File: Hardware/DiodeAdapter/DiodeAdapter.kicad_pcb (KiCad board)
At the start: 2 copper layers, 83 x 78 mm, 305 parts, among them P1 LED, P2 LED, P3 LED, P4 LED, X01 CONN_01X02, X02 CONN_01X02, X1 CONN_01X02, X2 CONN_01X02, X3 CONN_01X02, X4 CONN_01X02, X5 CONN_01X02, X6 CONN_01X02

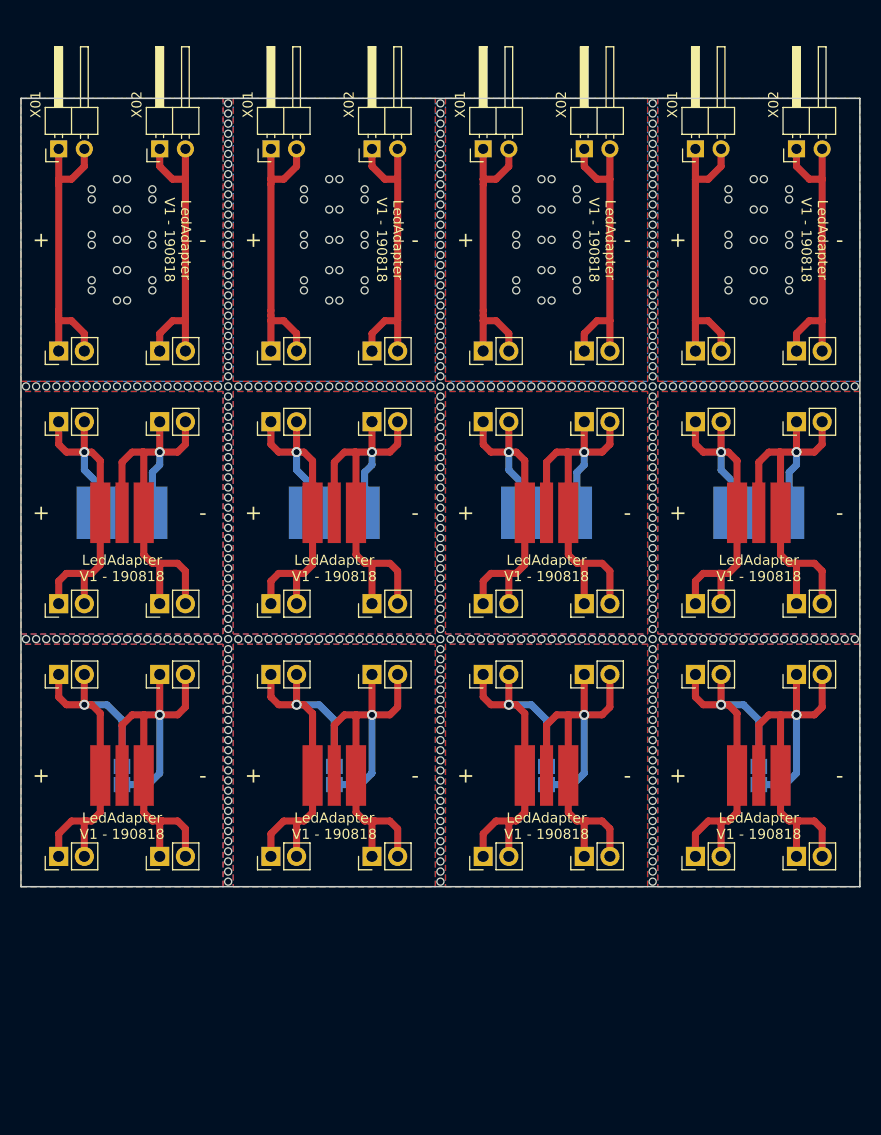
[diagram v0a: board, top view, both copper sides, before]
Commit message: Update for next version
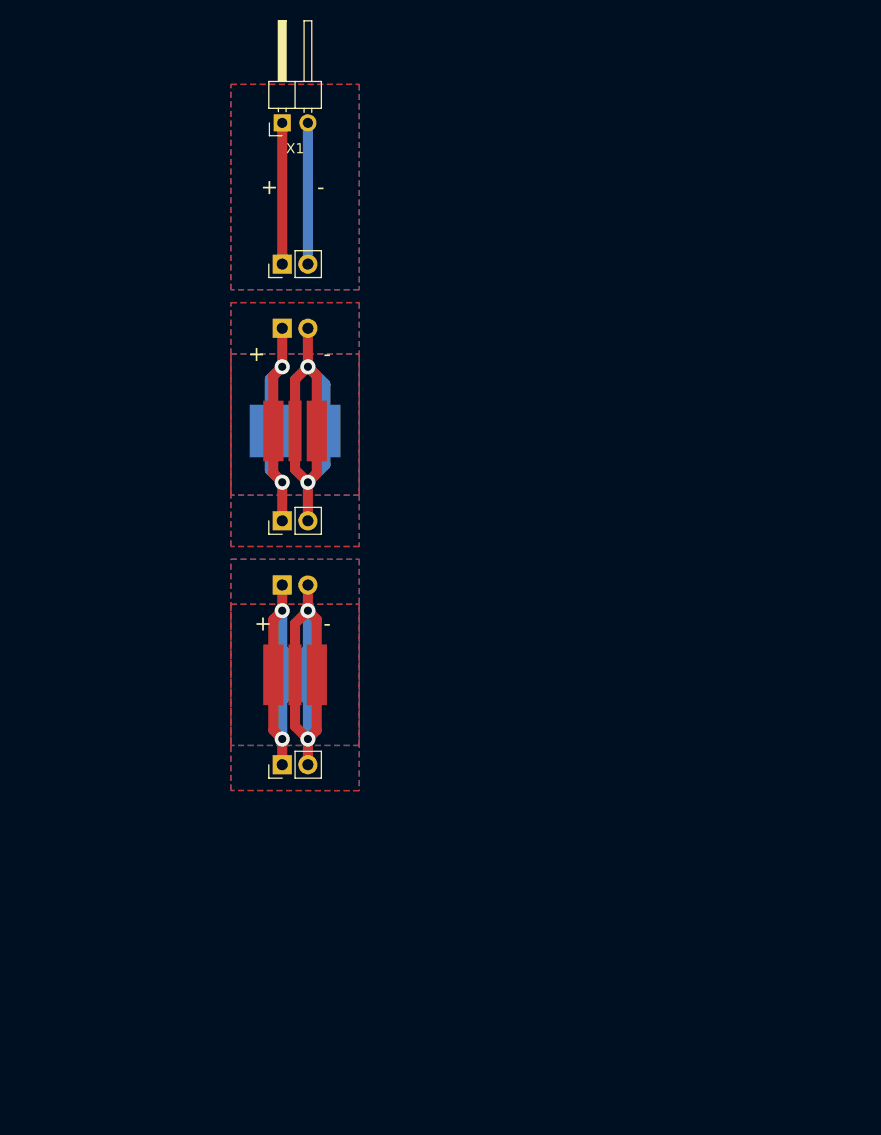
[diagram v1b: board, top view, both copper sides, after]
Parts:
- removed the P1 at (127.0, 87.0)
- removed the P1 at (106.0, 87.0)
- removed the P1 at (85.0, 87.0)
- removed the P1 at (64.0, 87.0)
- removed the P2 at (127.0, 87.0)
- removed the P2 at (106.0, 87.0)
- removed the P2 at (85.0, 87.0)
- removed the P2 at (64.0, 87.0)
- removed the P3 at (127.0, 113.0)
- removed the P3 at (106.0, 113.0)
- removed the P3 at (85.0, 113.0)
- removed the P3 at (64.0, 113.0)
- removed the P4 at (127.0, 113.0)
- removed the P4 at (106.0, 113.0)
- removed the P4 at (85.0, 113.0)
- removed the P4 at (64.0, 113.0)
- removed REF** (x241): BoardCutter_2, MyLib:BoardCutter_2
- removed X01 (x4), X02 (x4): CONN_01X02, MyLib:Pin_Header_Angled_1x02_Pitch2.54mm
- removed the X1 at (122.0, 71.0)
- removed the X1 at (101.0, 71.0)
- removed the X1 at (80.0, 71.0)
- removed the X1 at (59.0, 71.0)
- removed the X2 at (132.0, 71.0)
- removed the X2 at (111.0, 71.0)
- removed the X2 at (90.0, 71.0)
- removed the X2 at (69.0, 71.0)
- removed the X3 at (122.0, 78.0)
- removed the X3 at (122.0, 96.0)
- removed the X3 at (101.0, 96.0)
- removed the X3 at (101.0, 78.0)
- removed the X3 at (80.0, 78.0)
- removed the X3 at (80.0, 96.0)
- removed the X3 at (59.0, 96.0)
- removed the X3 at (59.0, 78.0)
- removed the X4 at (132.0, 78.0)
- removed the X4 at (132.0, 96.0)
- removed the X4 at (111.0, 96.0)
- removed the X4 at (111.0, 78.0)
- removed the X4 at (90.0, 78.0)
- removed the X4 at (90.0, 96.0)
- removed the X4 at (69.0, 96.0)
- removed the X4 at (69.0, 78.0)
- removed the X5 at (122.0, 103.0)
- removed the X5 at (122.0, 121.0)
- removed the X5 at (101.0, 121.0)
- removed the X5 at (101.0, 103.0)
- removed the X5 at (80.0, 103.0)
- removed the X5 at (80.0, 121.0)
- removed the X5 at (59.0, 121.0)
- removed the X5 at (59.0, 103.0)
- removed the X6 at (132.0, 103.0)
- removed the X6 at (132.0, 121.0)
- removed the X6 at (111.0, 121.0)
- removed the X6 at (111.0, 103.0)
- removed the X6 at (90.0, 103.0)
- removed the X6 at (90.0, 121.0)
- removed the X6 at (69.0, 121.0)
- removed the X6 at (69.0, 103.0)
- added P1: LED, 0EsseivaN_Lib:LED_LH351D, F.Cu at (81.1, 78.9)
- added P2: LED, 0EsseivaN_Lib:LED_LITTLE_STAR, B.Cu at (81.1, 78.9)
- added P3: LED, 0EsseivaN_Lib:LED_LH351D, F.Cu at (81.1, 103.0)
- added P4: LED, 0EsseivaN_Lib:LED_XQ_D, B.Cu at (81.1, 103.0)
- added X1: CONN_01X02, 0EsseivaN_Lib:Pin_Header_Angled_1x02_Pitch2.54mm, F.Cu at (81.1, 48.4)
- added X2: CONN_01X02, 0EsseivaN_Lib:Pin_Header_Straight_1x02_Pitch2.54mm, F.Cu at (81.1, 62.4)
- added X3: CONN_01X02, 0EsseivaN_Lib:Pin_Header_Straight_1x02_Pitch2.54mm, F.Cu at (81.1, 87.8)
- added X4: CONN_01X02, 0EsseivaN_Lib:Pin_Header_Straight_1x02_Pitch2.54mm, B.Cu at (81.1, 68.8)
- added X5: CONN_01X02, 0EsseivaN_Lib:Pin_Header_Straight_1x02_Pitch2.54mm, B.Cu at (81.1, 94.2)
- added X6: CONN_01X02, 0EsseivaN_Lib:Pin_Header_Straight_1x02_Pitch2.54mm, F.Cu at (81.1, 111.9)
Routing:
- net /GND_2: track 201.5 -> 45.3 mm, vias 4 -> 2
- net /GND_1: track 184.3 -> 45.1 mm, vias 4 -> 2
- net /V+_2: track 158.9 -> 31.5 mm, vias 4 -> 2
- net /V+_1: track 150.6 -> 32.2 mm, vias 4 -> 2
- net /V+: track 118.4 -> 14.0 mm
- net /GND: track 118.4 -> 14.0 mm
- added copper zone on F.Cu, net /GND_1
- added copper zone on F.Cu, net /GND_2
- removed copper zone on F.Cu, net /V+_1
- removed copper zone on F.Cu, net /V+_2
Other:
- board outline removed
- net class Default: trace_width 0.7 -> 1; via_dia 1 -> 1.5; via_drill 0.6 -> 0.8
- board text removed: "Holes to better stick with glue"
- board text removed: "LedAdapter V1 - 190818"

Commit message: Version 6 final
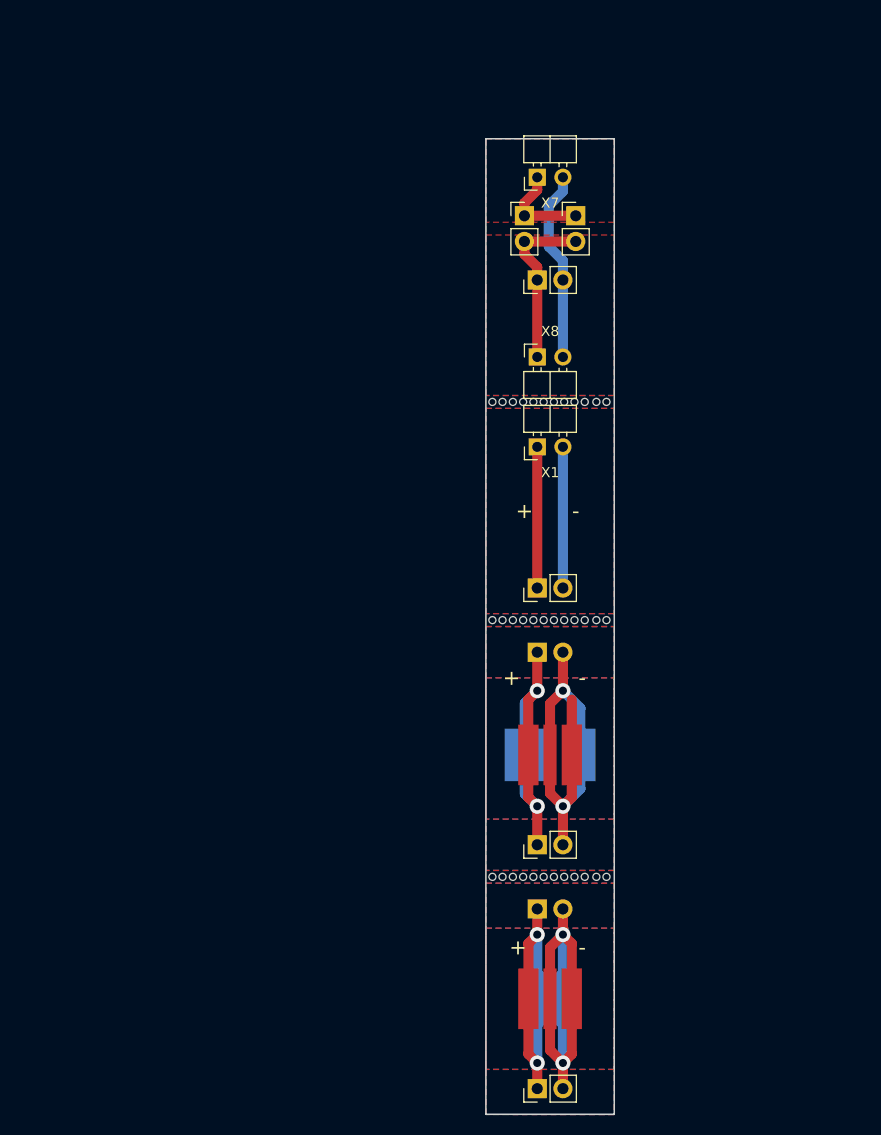
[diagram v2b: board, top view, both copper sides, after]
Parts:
- added REF**: BoardCutter_2, 0EsseivaN_Lib:BoardCutter_2, F.Cu at (111.4, 123.0)
- added REF**: BoardCutter_2, 0EsseivaN_Lib:BoardCutter_2, F.Cu at (111.4, 97.6)
- added REF**: BoardCutter_2, 0EsseivaN_Lib:BoardCutter_2, F.Cu at (111.4, 76.0)
- added REF**: BoardCutter_10, 0EsseivaN_Lib:BoardCutter_10, F.Cu at (100.6, 123.0)
- added REF**: BoardCutter_10, 0EsseivaN_Lib:BoardCutter_10, F.Cu at (100.6, 97.6)
- added REF**: BoardCutter_10, 0EsseivaN_Lib:BoardCutter_10, F.Cu at (100.6, 76.0)
- added W1: TEST_2P, 0EsseivaN_Lib:Pin_Header_Straight_1x02_Pitch2.54mm, F.Cu at (103.8, 58.9)
- added W2: TEST_2P, 0EsseivaN_Lib:Pin_Header_Straight_1x02_Pitch2.54mm, F.Cu at (108.9, 58.9)
- added X7: CONN_01X02, 0EsseivaN_Lib:Pin_Header_Angled_1x02_Pitch2.54mm, F.Cu at (106.3, 53.8)
- added X8: CONN_01X02, 0EsseivaN_Lib:Pin_Header_Angled_1x02_Pitch2.54mm_reverse, F.Cu at (106.3, 71.6)
- added X9: CONN_01X02, 0EsseivaN_Lib:Pin_Header_Straight_1x02_Pitch2.54mm, F.Cu at (106.3, 64.0)
- moved X1 40.8 mm to (106.3, 80.5)
- moved X2 40.8 mm to (106.3, 94.5)
- moved P1 40.8 mm to (106.3, 111.0)
- moved P2 40.8 mm to (106.3, 111.0)
- moved P3 40.8 mm to (106.3, 135.1)
- moved P4 40.8 mm to (106.3, 135.1), turned to 90 degrees
- moved X3 40.8 mm to (106.3, 119.8)
- moved X4 40.8 mm to (106.3, 100.8)
- moved X5 40.8 mm to (106.3, 126.2)
- moved X6 40.8 mm to (106.3, 144.0)
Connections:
- P1 pad 1: /V+_1 -> /GND_1
- P1 pad 2: /GND_1 -> /V+_1
- P2 pad 1: /V+_1 -> /GND_1
- P2 pad 2: /GND_1 -> /V+_1
- P3 pad 1: /V+_2 -> /GND_2
- P3 pad 2: /GND_2 -> /V+_2
- P4 pad 1: /V+_2 -> /GND_2
- P4 pad 2: /GND_2 -> /V+_2
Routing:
- net Net-(X7-Pad2): track 0.00 -> 18.9 mm
- net Net-(W1-Pad2): track 0.00 -> 17.0 mm
- net Net-(W1-Pad1): track 0.00 -> 9.42 mm
- net /GND_1: track 45.1 -> 43.9 mm
- added copper zone on F.Cu, net Net-(W1-Pad1)
- added copper zone on F.Cu, net Net-(W1-Pad2)
- added copper zone on B.Cu, net Net-(X7-Pad2)
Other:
- board outline added: 12.7 x 96.5 mm
